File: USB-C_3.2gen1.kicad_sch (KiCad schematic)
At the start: 0 parts

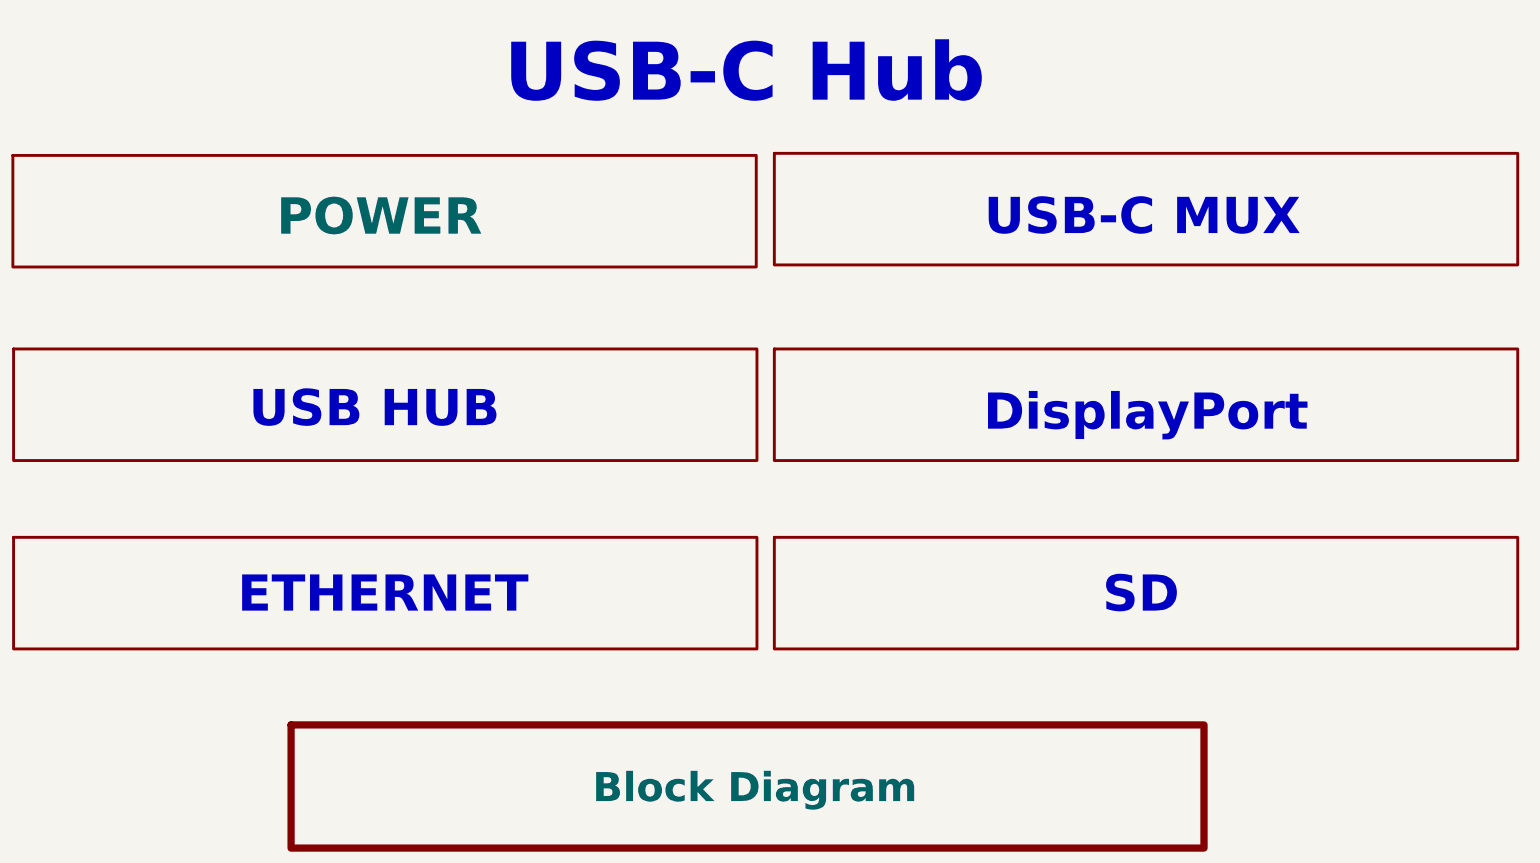
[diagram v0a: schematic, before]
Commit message: Add files via upload
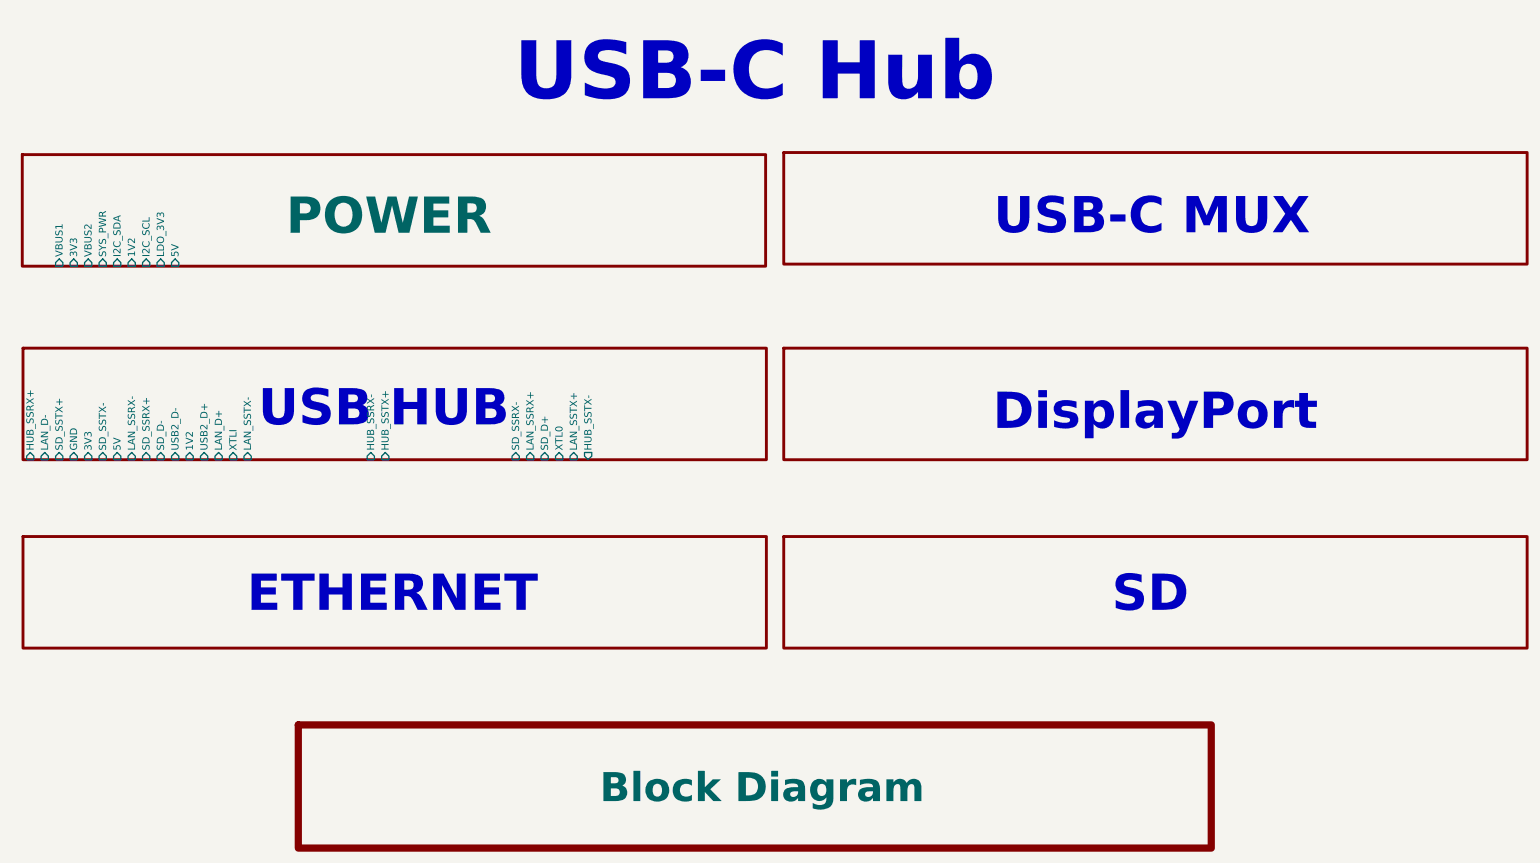
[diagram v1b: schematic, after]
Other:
- sheet POWER ports: added 1V2, 3V3, 5V, I2C_SCL, I2C_SDA, LDO_3V3, SYS_PWR, VBUS1, VBUS2; removed none
- sheet USB HUB ports: added 1V2, 3V3, 5V, GND, HUB_SSRX+, HUB_SSRX-, HUB_SSTX+, HUB_SSTX-, LAN_D+, LAN_D-, LAN_SSRX+, LAN_SSRX-, LAN_SSTX+, LAN_SSTX-, SD_D+, SD_D-, SD_SSRX+, SD_SSRX-, SD_SSTX+, SD_SSTX-, USB2_D+, USB2_D-, XTL0, XTLI; removed none
